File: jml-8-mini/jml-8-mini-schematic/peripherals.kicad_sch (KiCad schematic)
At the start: 9 parts, among them J2 SIO CHB, J3 UART, J4 CTC Extra Lines, U4 Z80 CTC, U5 Z80 SIO

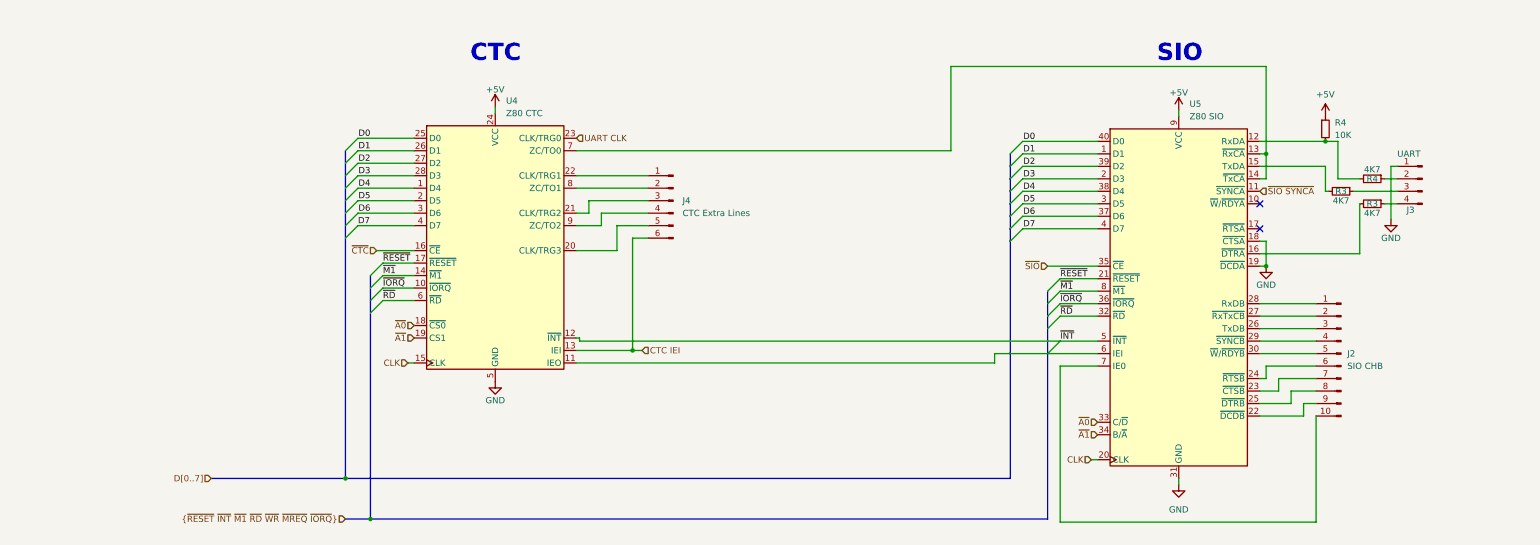
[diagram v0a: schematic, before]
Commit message: lots of updates to schematic to make pcb routing easier, start on pcb design
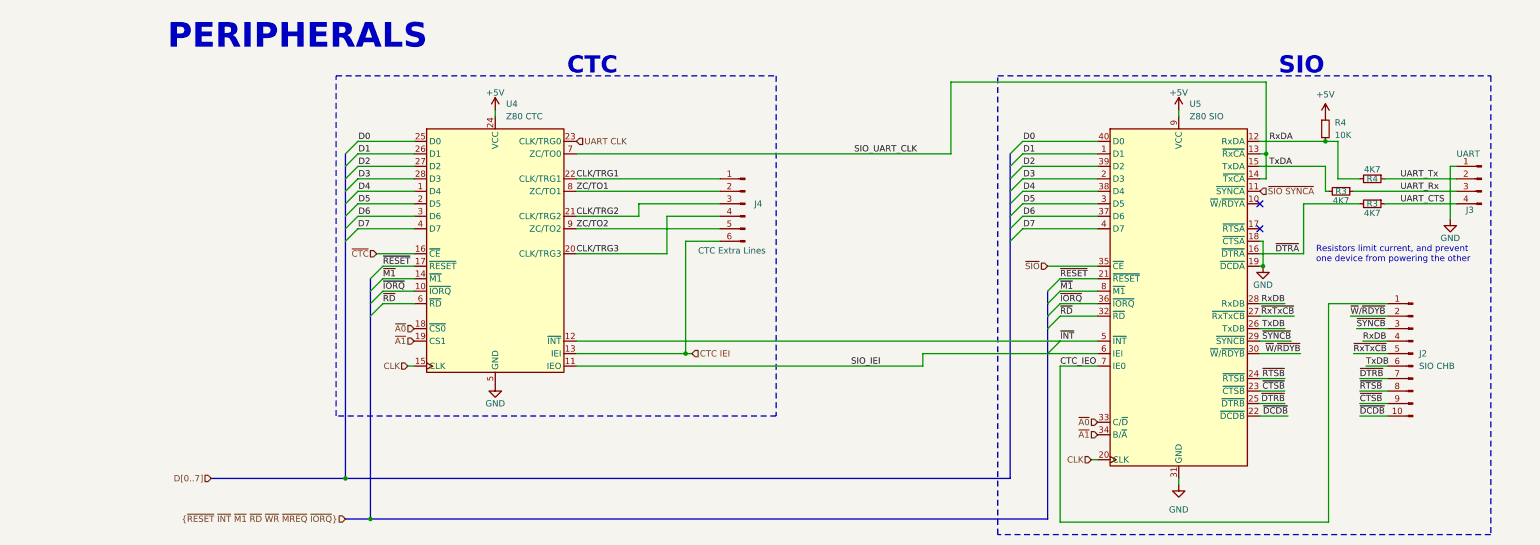
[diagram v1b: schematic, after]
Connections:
- net UART_CTS: now reaches J3.4 (Pin_4), R3.1
- net ~{DTRA}: now reaches R3.2, U5.16 (~{DTRA})
- net UART_Tx: now reaches J3.2 (Pin_2), R4.1
- net RxDA: now reaches R4.2, R4.2, U5.12 (RxDA)
- net CLK/TRG1: now reaches J4.1 (Pin_1), U4.22 (CLK/TRG1)
- net ZC/TO1: now reaches J4.2 (Pin_2), U4.8 (ZC/TO1)
- net CLK/TRG2: now reaches J4.3 (Pin_3), U4.21 (CLK/TRG2)
- net CLK/TRG3: now reaches J4.4 (Pin_4)
- net CLK/TRG3: now also U4.20 (CLK/TRG3); no longer U4.9 (ZC/TO2)
- net ZC/TO2: now reaches J4.5 (Pin_5)
- net ZC/TO2: now also U4.9 (ZC/TO2); no longer U4.20 (CLK/TRG3)
- net UART_Rx: now reaches J3.3 (Pin_3), R3.1
- net TxDA: now reaches R3.2, U5.15 (TxDA)
- net CTC_IEO: now reaches J2.1 (Pin_1)
- net CTC_IEO: now also U5.7 (IE0); no longer U5.28 (RxDB)
- net ~{DCDB}: now reaches J2.10 (Pin_10)
- net ~{DCDB}: now also U5.22 (~{DCDB}); no longer U5.7 (IE0)
- net ~{RxTxCB}: now reaches U5.27 (~{RxTxCB})
- net ~{RxTxCB}: now also J2.5 (Pin_5); no longer J2.2 (Pin_2)
- net TxDB: now reaches U5.26 (TxDB)
- net TxDB: now also J2.6 (Pin_6); no longer J2.3 (Pin_3)
- net RxDB: now reaches J2.4 (Pin_4)
- net RxDB: now also U5.28 (RxDB); no longer U5.29 (~{SYNCB})
- net ~{W}/~{RDYB}: now reaches U5.30 (~{W}/~{RDYB})
- net ~{W}/~{RDYB}: now also J2.2 (Pin_2); no longer J2.5 (Pin_5)
- net ~{RTSB}: now reaches U5.24 (~{RTSB})
- net ~{RTSB}: now also J2.8 (Pin_8); no longer J2.6 (Pin_6)
- net ~{CTSB}: now reaches U5.23 (~{CTSB})
- net ~{CTSB}: now also J2.9 (Pin_9); no longer J2.7 (Pin_7)
- net ~{DTRB}: now reaches U5.25 (~{DTRB})
- net ~{DTRB}: now also J2.7 (Pin_7); no longer J2.8 (Pin_8)
- net SIO_UART_CLK: now reaches U4.7 (ZC/TO0), U5.13 (~{RxCA}), U5.14 (~{TxCA})
- net SIO_IEI: now reaches U4.11 (IEO), U5.6 (IEI)
- new net ~{SYNCB}: J2.3 (Pin_3), U5.29 (~{SYNCB})
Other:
- note added: "PERIPHERALS"
- note added: "Resistors limit current, and prevent one device from powering the other"
- moved on the sheet: J2, J3, J4, U4
